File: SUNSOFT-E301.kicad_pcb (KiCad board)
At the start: 2 copper layers, 92.1 x 57.1 mm, 27 parts, among them J1 Famicom Card Edge Connector, U1 HM6264, U2 FME7-5A-5B, U3 27C040, U4 27C020

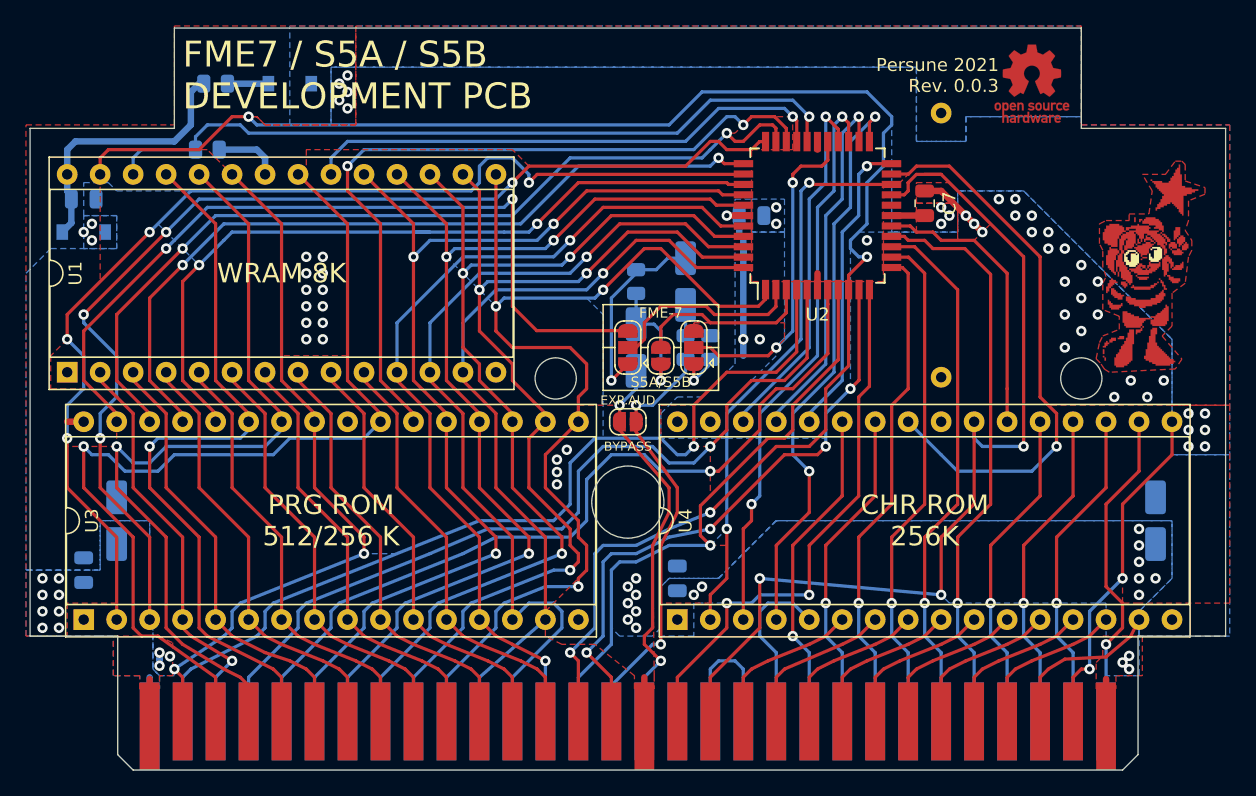
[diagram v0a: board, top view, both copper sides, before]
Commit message: KiCad 6.0
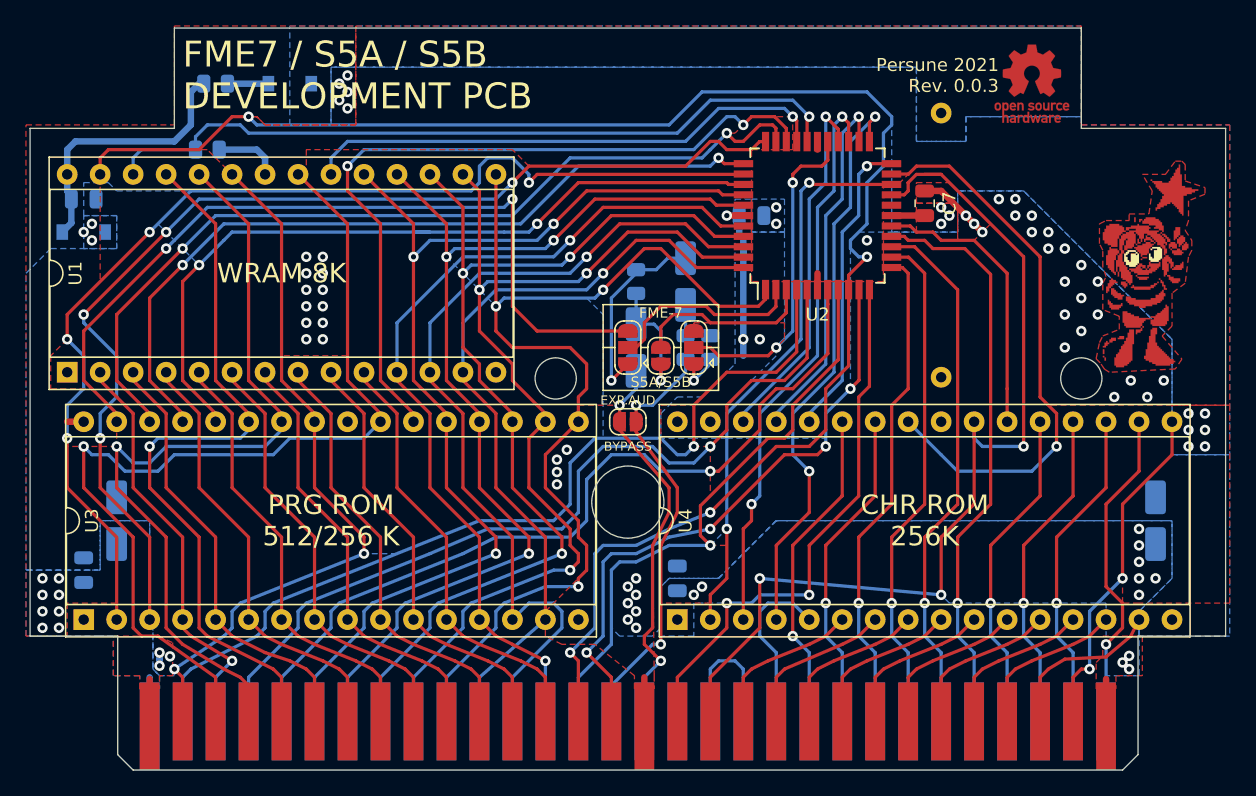
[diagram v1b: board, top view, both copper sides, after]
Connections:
- net /CHR_~CE renamed /CHR_~{CE}
- net /CPU_R~W renamed /CPU_R~{W}
- net /PPU_~RD renamed /PPU_~{RD}
- net /PRG_~CE renamed /PRG_~{CE}
- net /WRAM_~CE renamed /WRAM_~{CE}
- net /~IRQ renamed /~{IRQ}
- net /~ROMSEL renamed /~{ROMSEL}
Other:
- net class Default removed
- net class Power removed
